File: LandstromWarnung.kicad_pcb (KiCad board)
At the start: 4 copper layers, 40 x 60 mm, 19 parts, among them J10 K15 -, J11 Summer +, J3 Summer -, J7 Landstr. +, J8 Landstr. -, J9 K15 +, Q2 IRF7404, U5 LTV-847

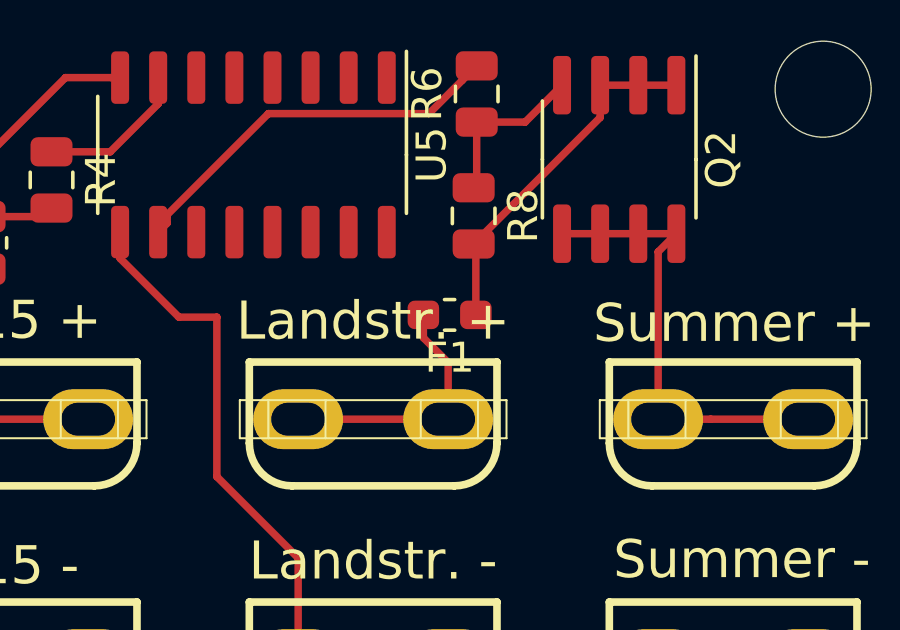
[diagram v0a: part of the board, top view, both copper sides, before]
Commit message: x
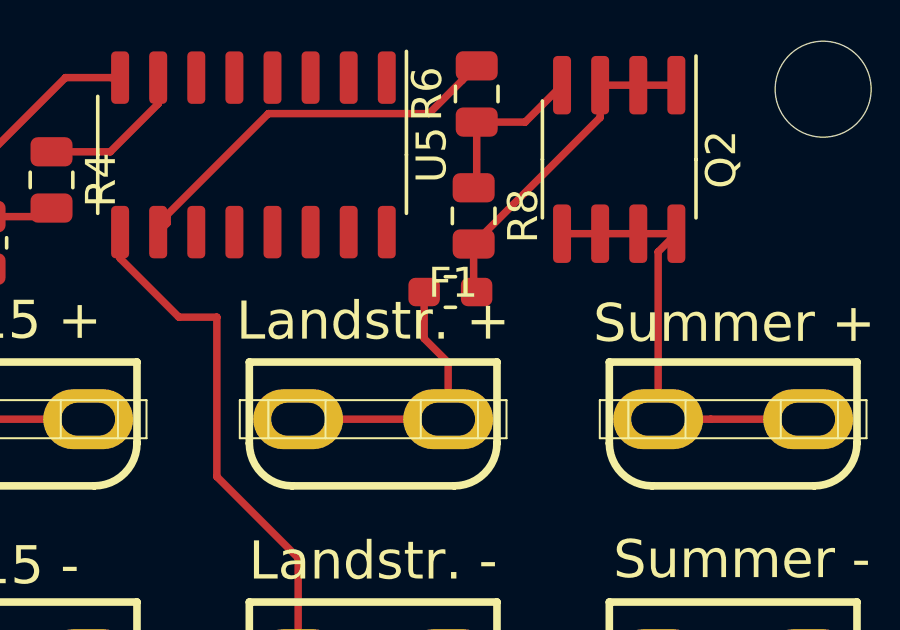
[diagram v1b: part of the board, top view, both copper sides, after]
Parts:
- moved F1 0.76 mm to (32.6, 19.8)
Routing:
- net Net-(F1-Pad2): track 8.82 -> 9.57 mm
- net +12V: track 12.0 -> 11.3 mm
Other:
- copper layers 4 -> 2
